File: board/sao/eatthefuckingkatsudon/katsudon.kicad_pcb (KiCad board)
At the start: 2 copper layers, 48.9 x 49.8 mm, 4 parts

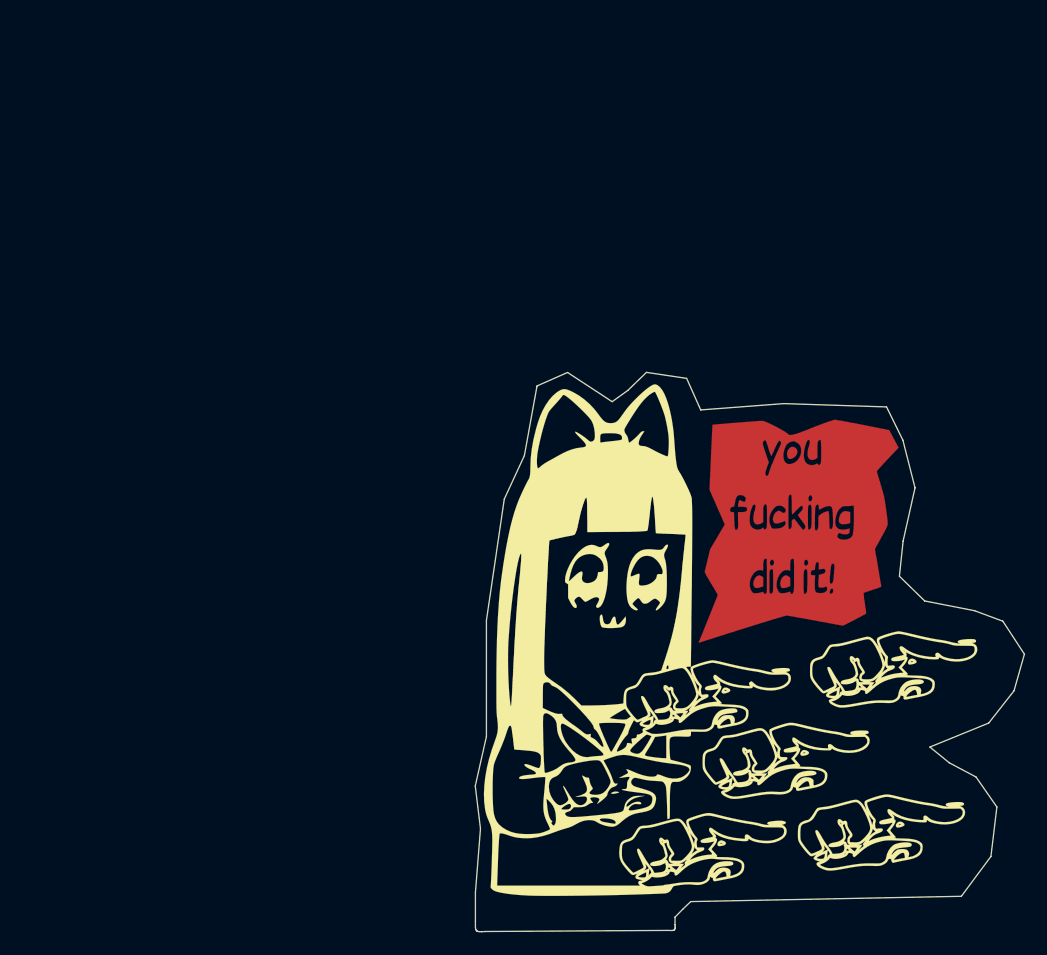
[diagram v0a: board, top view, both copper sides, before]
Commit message: work on punching popuko sao
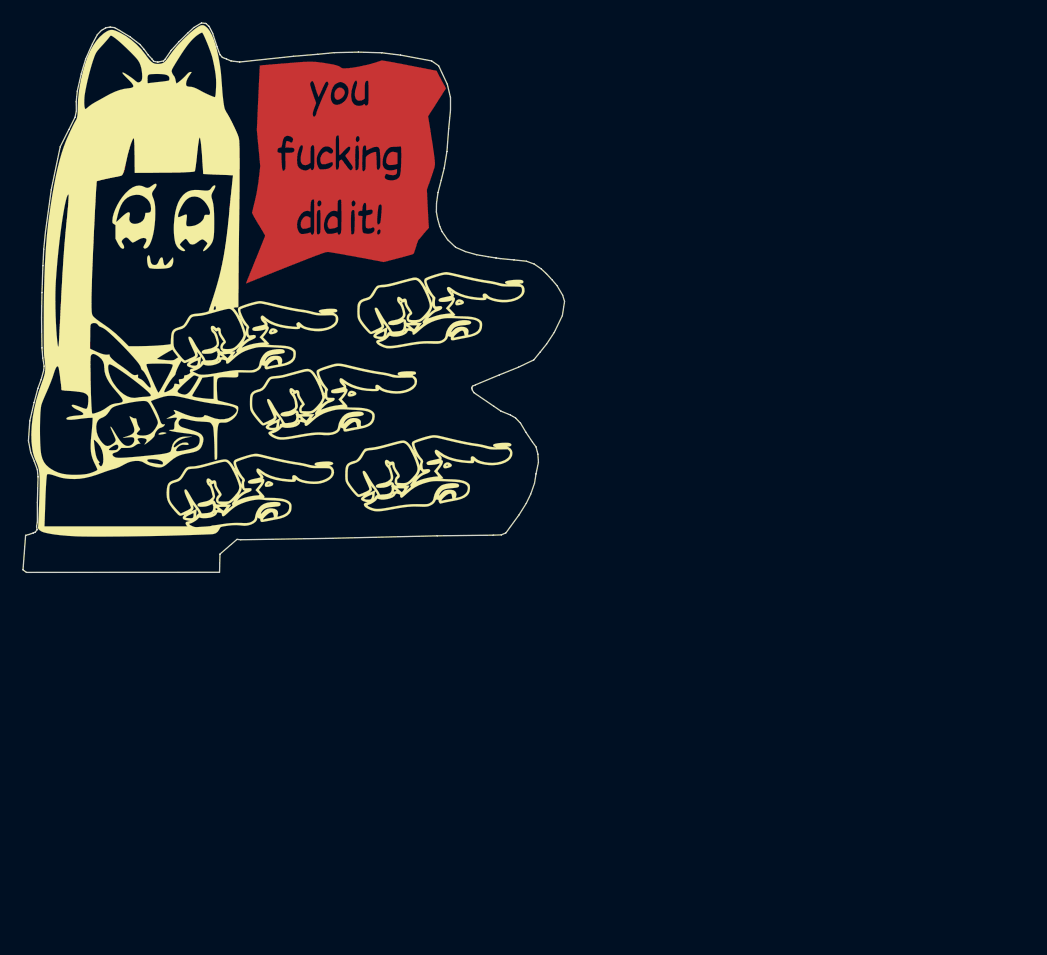
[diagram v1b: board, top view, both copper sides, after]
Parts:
- removed the G*** at (90.6, 73.6) (x4)
- added G*** (x4): LOGO, LOGO, F.Cu at (50.3, 41.6)
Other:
- board size 48.9 x 49.8 mm -> 48.2 x 48.9 mm
